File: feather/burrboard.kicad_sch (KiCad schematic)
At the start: 30 parts, among them J1 J1, J2 J2, J3 Conn_01x02_Male, Q1 TEMT6000X01, U1 TMP36, U2 ADXL345BCCZ

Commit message: Fixup
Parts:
- S1, S2: symbol dk_Tactile-Switches:PTS645SM43SMTR92_LFS -> burrboard:PTS645SM43SMTR92_LFS
- U2: footprint digikey-footprints:LGA-14_3x5mm_RevA -> burrboard:LGA-14_3x5mm_RevA
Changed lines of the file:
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@@
       (effects (font (size 1.524 1.524)) (justify left))
     )
-    (property "Footprint" "digikey-footprints:LGA-14_3x5mm_RevA" (id 2) (at 74.93 151.13 0)
+    (property "Footprint" "burrboard:LGA-14_3x5mm_RevA" (id 2) (at 74.93 151.13 0)
       (effects (font (size 1.524 1.524)) (justify left) hide)
     )
@@
     (pin "1")
   )
-  (symbol (lib_id "dk_Tactile-Switches:PTS645SM43SMTR92_LFS") (at 139.7 92.71 0) (unit 1)
+  (symbol (lib_id "burrboard:PTS645SM43SMTR92_LFS") (at 139.7 92.71 0) (unit 1)
     (in_bom yes) (on_board yes)
     (property "Reference" "S1" (id 0) (at 139.7 83.8962 0)
@@
     (pin "4")
   )
-  (symbol (lib_id "dk_Tactile-Switches:PTS645SM43SMTR92_LFS") (at 139.7 120.65 0) (unit 1)
+  (symbol (lib_id "burrboard:PTS645SM43SMTR92_LFS") (at 139.7 120.65 0) (unit 1)
     (in_bom yes) (on_board yes)
     (property "Reference" "S2" (id 0) (at 139.7 111.8362 0)
@@
     )
     (path "/00000000-0000-0000-0000-000061d5dad5"
-      (reference "U2") (unit 1) (value "ADXL345BCCZ") (footprint "digikey-footprints:LGA-14_3x5mm_RevA")
-    )
-  )
+      (reference "U2") (unit 1) (value "ADXL345BCCZ") (footprint "burrboard:LGA-14_3x5mm_RevA")
+    )
+  )

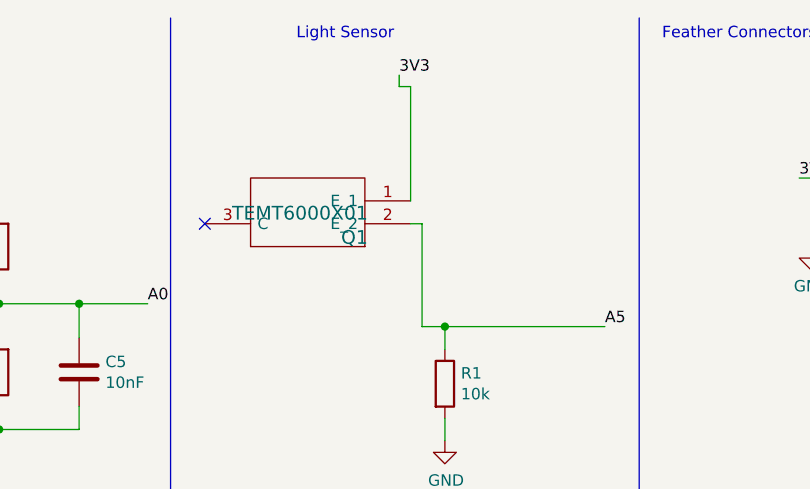
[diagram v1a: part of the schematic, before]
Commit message: Update
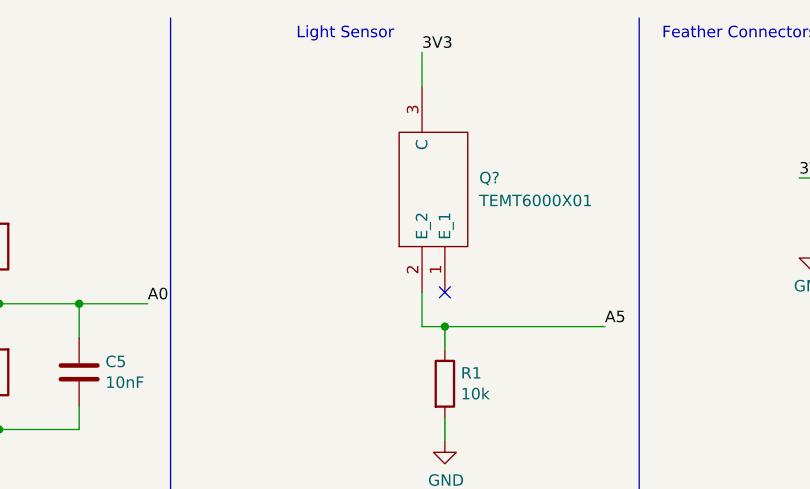
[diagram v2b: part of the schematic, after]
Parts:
- removed Q1: TEMT6000X01, burrboard:Phototransistor_SMD_4x2mm_TEMT6000X01, symbol burrboard:TEMT6000X01
- added Q?: TEMT6000X01, burrboard:Phototransistor_SMD_4x2mm_TEMT6000X01, symbol burrboard:TEMT6000X01
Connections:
- net 3V3: now also Q?.3 (C)
- net A5: now also Q?.2 (E_2)
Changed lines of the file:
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@@
   (no_connect (at 134.62 95.25))
   (no_connect (at 229.87 60.96))
-  (no_connect (at 153.67 35.56))
+  (no_connect (at 180.34 43.18))
   (no_connect (at 229.87 33.02))
   (no_connect (at 229.87 66.04))
@@
     (stroke (width 0) (type default) (color 0 0 0 0))
   )
-  (wire (pts (xy 175.26 20.32) (xy 175.26 19.05))
-    (stroke (width 0) (type default) (color 0 0 0 0))
-  )
   (wire (pts (xy 132.08 172.72) (xy 134.62 172.72))
     (stroke (width 0) (type default) (color 0 0 0 0))
@@
     (stroke (width 0) (type default) (color 0 0 0 0))
   )
+  (wire (pts (xy 177.8 43.18) (xy 177.8 46.99))
+    (stroke (width 0) (type default) (color 0 0 0 0))
+  )
   (wire (pts (xy 109.22 30.48) (xy 130.81 30.48))
     (stroke (width 0) (type default) (color 0 0 0 0))
@@
     (stroke (width 0) (type default) (color 0 0 0 0))
   )
-  (wire (pts (xy 177.8 35.56) (xy 176.53 35.56))
-    (stroke (width 0) (type default) (color 0 0 0 0))
-  )
   (wire (pts (xy 55.88 62.23) (xy 55.88 66.04))
     (stroke (width 0) (type default) (color 0 0 0 0))
@@
     (stroke (width 0) (type default) (color 0 0 0 0))
   )
+  (wire (pts (xy 177.8 16.51) (xy 177.8 20.32))
+    (stroke (width 0) (type default) (color 0 0 0 0))
+  )
   (wire (pts (xy 229.87 43.18) (xy 224.79 43.18))
     (stroke (width 0) (type default) (color 0 0 0 0))
@@
     (stroke (width 0) (type default) (color 0 0 0 0))
   )
-  (wire (pts (xy 176.53 20.32) (xy 175.26 20.32))
-    (stroke (width 0) (type default) (color 0 0 0 0))
-  )
   (wire (pts (xy 273.05 132.08) (xy 273.05 143.51))
     (stroke (width 0) (type default) (color 0 0 0 0))
@@
     (stroke (width 0) (type default) (color 0 0 0 0))
   )
-  (wire (pts (xy 177.8 35.56) (xy 177.8 46.99))
-    (stroke (width 0) (type default) (color 0 0 0 0))
-  )
   (polyline (pts (xy 96.52 76.2) (xy 73.66 76.2))
     (stroke (width 0) (type default) (color 0 0 0 0))
@@
   )
   (wire (pts (xy 39.37 156.21) (xy 39.37 149.86))
-    (stroke (width 0) (type default) (color 0 0 0 0))
-  )
-  (wire (pts (xy 176.53 33.02) (xy 176.53 20.32))
     (stroke (width 0) (type default) (color 0 0 0 0))
   )
@@
     (effects (font (size 1.27 1.27)) (justify left bottom))
   )
-  (label "3V3" (at 175.26 19.05 0)
+  (label "3V3" (at 177.8 16.51 0)
     (effects (font (size 1.27 1.27)) (justify left bottom))
   )
@@
     (pin "2")
   )
-  (symbol (lib_id "burrboard:TEMT6000X01") (at 176.53 35.56 180) (unit 1)
-    (in_bom yes) (on_board yes)
-    (property "Reference" "Q1" (id 0) (at 171.7802 37.084 0)
-      (effects (font (size 1.524 1.524)) (justify left))
-    )
-    (property "Value" "TEMT6000X01" (id 1) (at 171.7802 34.3916 0)
-      (effects (font (size 1.524 1.524)) (justify left))
-    )
-    (property "Footprint" "burrboard:Phototransistor_SMD_4x2mm_TEMT6000X01" (id 2) (at 157.48 38.1 0)
-      (effects (font (size 1.27 1.27)) (justify left) hide)
-    )
-    (property "Datasheet" "https://www.vishay.com/docs/81579/temt6000.pdf" (id 3) (at 157.48 35.56 0)
-      (effects (font (size 1.27 1.27)) (justify left) hide)
-    )
-    (property "Digi-Key_PN" "751-1055-1-ND" (id 4) (at 171.45 45.72 0)
-      (effects (font (size 1.524 1.524)) (justify left) hide)
-    )
-    (property "MPN" "TEMT6000X01" (id 5) (at 171.45 48.26 0)
-      (effects (font (size 1.524 1.524)) (justify left) hide)
-    )
-    (property "Category" "Sensors, Transducers" (id 6) (at 171.45 50.8 0)
-      (effects (font (size 1.524 1.524)) (justify left) hide)
-    )
-    (property "Family" "Optical Sensors - Phototransistors" (id 7) (at 171.45 53.34 0)
-      (effects (font (size 1.524 1.524)) (justify left) hide)
-    )
-    (property "DK_Datasheet_Link" "http://www.vishay.com/docs/81579/temt6000.pdf" (id 8) (at 171.45 55.88 0)
-      (effects (font (size 1.524 1.524)) (justify left) hide)
-    )
-    (property "DK_Detail_Page" "/product-detail/en/vishay-semiconductor-opto-division/TEMT6000X01/751-1055-1-ND/1681410" (id 9) (at 171.45 58.42 0)
-      (effects (font (size 1.524 1.524)) (justify left) hide)
-    )
-    (property "Description" "Ambient Light Sensor 570nm SMD3 Vishay TEMT6000X01 +/-60  Visible Light Phototransistor, Surface Mount 3-Pin 1206 package" (id 10) (at 157.48 33.02 0)
-      (effects (font (size 1.27 1.27)) (justify left) hide)
-    )
-    (property "Manufacturer" "Vishay Semiconductor Opto Division" (id 11) (at 171.45 63.5 0)
-      (effects (font (size 1.524 1.524)) (justify left) hide)
-    )
-    (property "Status" "Active" (id 12) (at 171.45 66.04 0)
-      (effects (font (size 1.524 1.524)) (justify left) hide)
-    )
-    (property "AISLER_MPN" "TEMT6000X01" (id 13) (at 176.53 35.56 0)
-      (effects (font (size 1.27 1.27)) hide)
-    )
-    (property "Height" "" (id 14) (at 157.48 30.48 0)
-      (effects (font (size 1.27 1.27)) (justify left) hide)
-    )
-    (property "Manufacturer_Name" "Vishay" (id 15) (at 157.48 27.94 0)
-      (effects (font (size 1.27 1.27)) (justify left) hide)
-    )
-    (property "Manufacturer_Part_Number" "TEMT6000X01" (id 16) (at 157.48 25.4 0)
-      (effects (font (size 1.27 1.27)) (justify left) hide)
-    )
-    (property "Mouser Part Number" "78-TEMT6000" (id 17) (at 157.48 22.86 0)
-      (effects (font (size 1.27 1.27)) (justify left) hide)
-    )
-    (property "Mouser Price/Stock" "https://www.mouser.co.uk/ProductDetail/Vishay-Semiconductors/TEMT6000X01?qs=%2Fjqivxn91ccZGXDwz0wGxg%3D%3D" (id 18) (at 157.48 20.32 0)
-      (effects (font (size 1.27 1.27)) (justify left) hide)
-    )
-    (property "Arrow Part Number" "TEMT6000X01" (id 19) (at 157.48 17.78 0)
-      (effects (font (size 1.27 1.27)) (justify left) hide)
-    )
-    (property "Arrow Price/Stock" "https://www.arrow.com/en/products/temt6000x01/vishay?region=nac" (id 20) (at 157.48 15.24 0)
-      (effects (font (size 1.27 1.27)) (justify left) hide)
-    )
-    (pin "1")
-    (pin "2")
-    (pin "3")
-  )
   (symbol (lib_id "Switch:SW_SPDT") (at 148.59 185.42 0) (unit 1)
     (in_bom yes) (on_board yes)
@@
     (pin "2")
   )
+  (symbol (lib_id "burrboard:TEMT6000X01") (at 177.8 43.18 90) (unit 1)
+    (in_bom yes) (on_board yes) (fields_autoplaced)
+    (property "Reference" "Q?" (id 0) (at 184.15 30.4799 90)
+      (effects (font (size 1.27 1.27)) (justify right))
+    )
+    (property "Value" "TEMT6000X01" (id 1) (at 184.15 33.0199 90)
+      (effects (font (size 1.27 1.27)) (justify right))
+    )
+    (property "Footprint" "burrboard:Phototransistor_SMD_4x2mm_TEMT6000X01" (id 2) (at 175.26 24.13 0)
+      (effects (font (size 1.27 1.27)) (justify left) hide)
+    )
+    (property "Datasheet" "https://www.vishay.com/docs/81579/temt6000.pdf" (id 3) (at 177.8 24.13 0)
+      (effects (font (size 1.27 1.27)) (justify left) hide)
+    )
+    (property "Description" "Ambient Light Sensor 570nm SMD3 Vishay TEMT6000X01 +/-60  Visible Light Phototransistor, Surface Mount 3-Pin 1206 package" (id 4) (at 180.34 24.13 0)
+      (effects (font (size 1.27 1.27)) (justify left) hide)
+    )
+    (property "Height" "" (id 5) (at 182.88 24.13 0)
+      (effects (font (size 1.27 1.27)) (justify left) hide)
+    )
+    (property "Manufacturer_Name" "Vishay" (id 6) (at 185.42 24.13 0)
+      (effects (font (size 1.27 1.27)) (justify left) hide)
+    )
+    (property "Manufacturer_Part_Number" "TEMT6000X01" (id 7) (at 187.96 24.13 0)
+      (effects (font (size 1.27 1.27)) (justify left) hide)
+    )
+    (property "Mouser Part Number" "78-TEMT6000" (id 8) (at 190.5 24.13 0)
+      (effects (font (size 1.27 1.27)) (justify left) hide)
+    )
+    (property "Mouser Price/Stock" "https://www.mouser.co.uk/ProductDetail/Vishay-Semiconductors/TEMT6000X01?qs=%2Fjqivxn91ccZGXDwz0wGxg%3D%3D" (id 9) (at 193.04 24.13 0)
+      (effects (font (size 1.27 1.27)) (justify left) hide)
+    )
+    (property "Arrow Part Number" "TEMT6000X01" (id 10) (at 195.58 24.13 0)
+      (effects (font (size 1.27 1.27)) (justify left) hide)
+    )
+    (property "Arrow Price/Stock" "https://www.arrow.com/en/products/temt6000x01/vishay?region=nac" (id 11) (at 198.12 24.13 0)
+      (effects (font (size 1.27 1.27)) (justify left) hide)
+    )
+    (pin "1")
+    (pin "2")
+    (pin "3")
+  )
   (symbol (lib_id "Device:C") (at 139.7 52.07 0) (unit 1)
     (in_bom yes) (on_board yes)
@@
       (reference "J3") (unit 1) (value "Conn_01x02_Male") (footprint "Connector_PinHeader_2.54mm:PinHeader_1x02_P2.54mm_Vertical")
     )
-    (path "/00000000-0000-0000-0000-000061ecf6dc"
-      (reference "Q1") (unit 1) (value "TEMT6000X01") (footprint "burrboard:Phototransistor_SMD_4x2mm_TEMT6000X01")
+    (path "/666dc925-2b95-4de4-a148-45e51fb4be3f"
+      (reference "Q?") (unit 1) (value "TEMT6000X01") (footprint "burrboard:Phototransistor_SMD_4x2mm_TEMT6000X01")
     )
     (path "/00000000-0000-0000-0000-000061c212d9"
